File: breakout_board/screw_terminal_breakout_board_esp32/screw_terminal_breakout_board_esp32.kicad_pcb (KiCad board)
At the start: 2 copper layers, 75 x 81 mm, 9 parts, among them J1 Screw_Terminal_01x15, J2 Screw_Terminal_01x15, J3 Conn_01x15_Socket, J4 Conn_01x15_Socket, U1 ESP32_DevKit_V1_DOIT

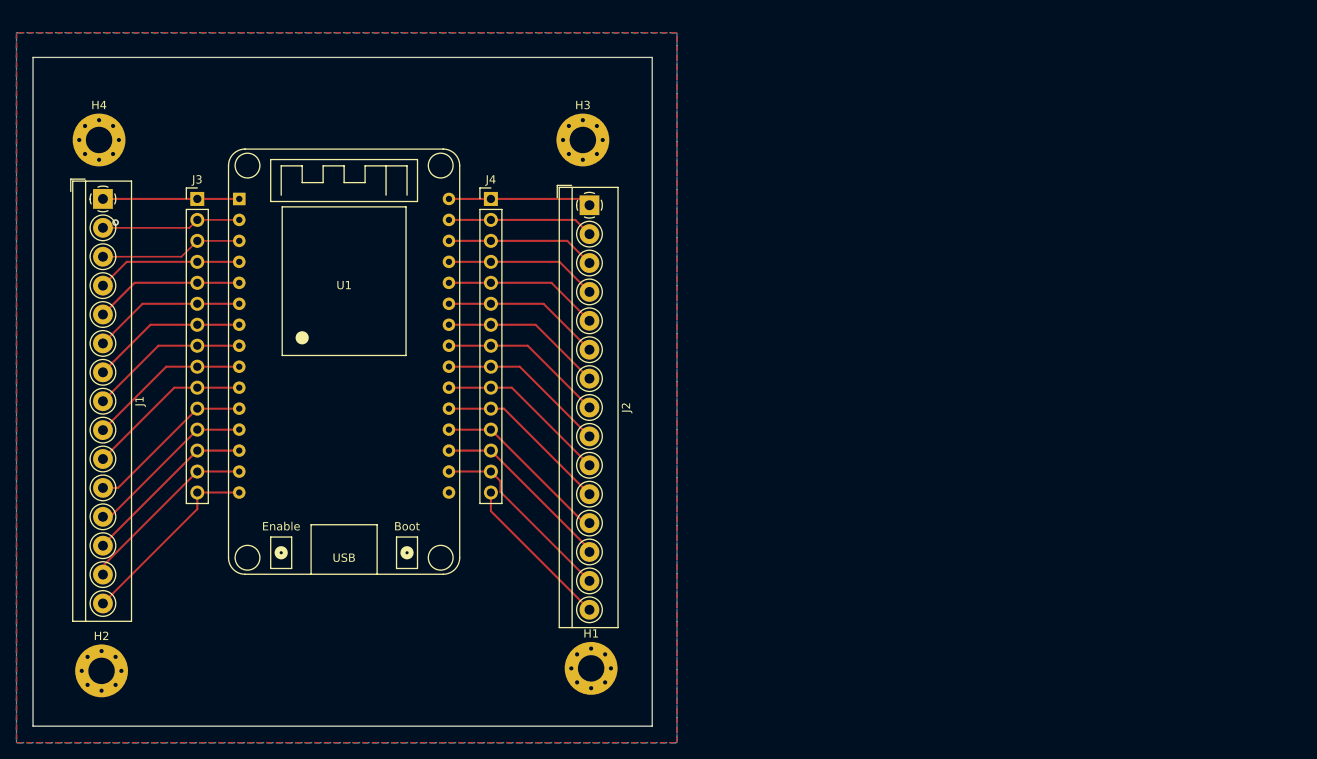
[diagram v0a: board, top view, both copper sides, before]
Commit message: pcb update
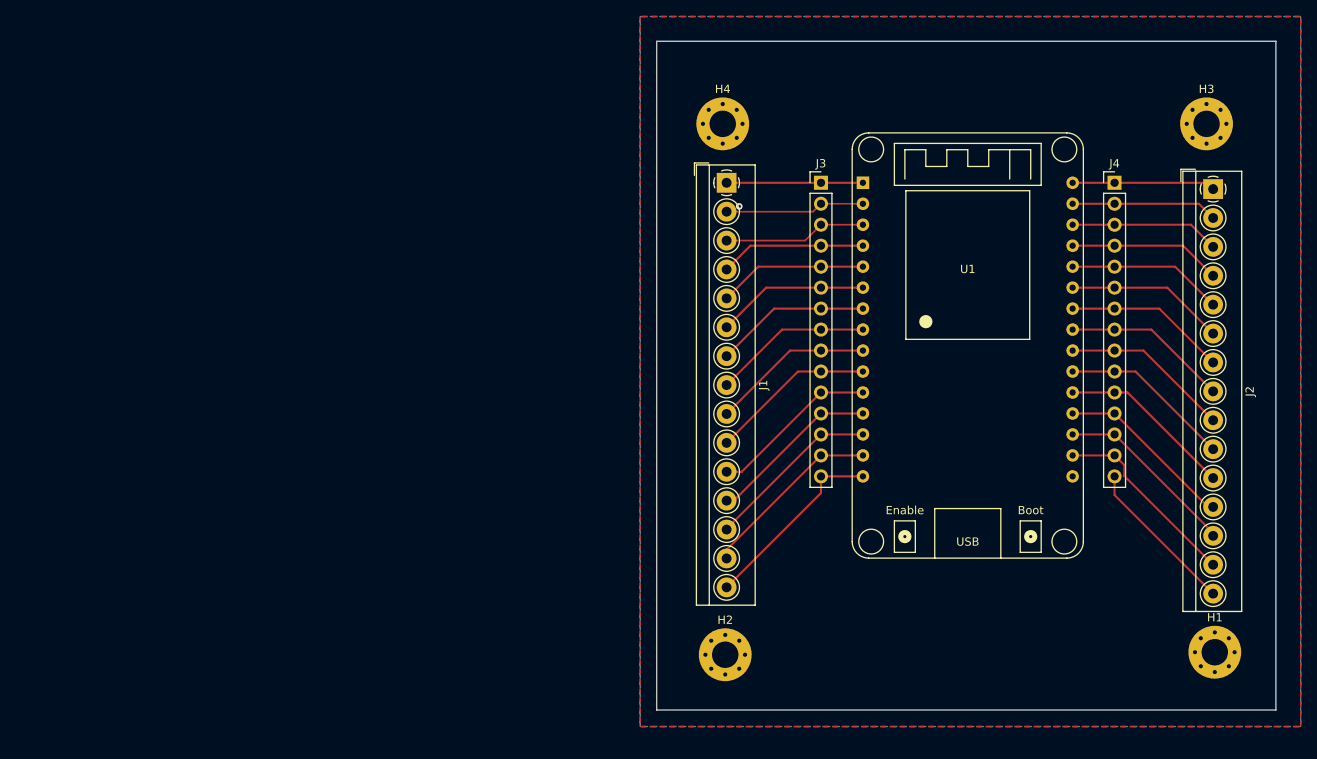
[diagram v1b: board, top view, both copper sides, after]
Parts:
- moved H1 75.6 mm to (169.7, 124.1)
- moved H3 75.6 mm to (168.7, 60.1)
- moved J2 75.6 mm to (169.5, 68.0)
- moved J3 75.6 mm to (122.0, 67.2)
- moved H2 75.6 mm to (110.4, 124.4)
- moved H4 75.6 mm to (110.1, 60.1)
- moved J1 75.6 mm to (110.5, 67.2)
- moved J4 75.6 mm to (157.5, 67.2)
- moved U1 75.6 mm to (139.8, 67.2)
